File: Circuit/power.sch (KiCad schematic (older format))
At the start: 19 parts, among them Q202 FDN340P, Q203 FDN340P, SW1 ON/OFF, U201 CN3063, U202 MCP6002

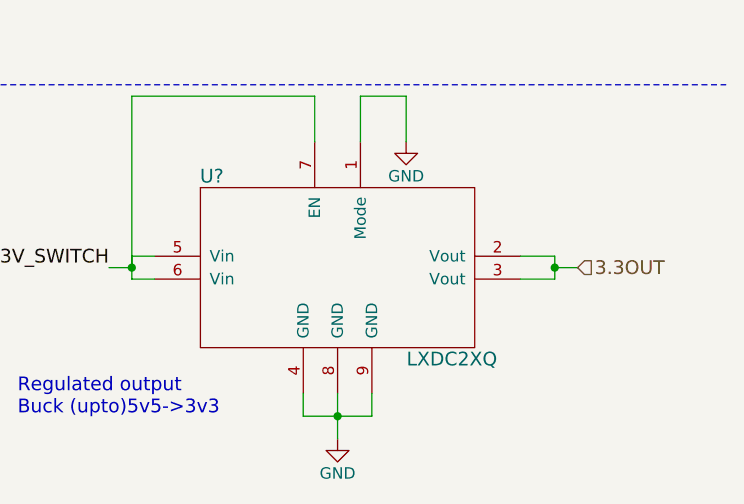
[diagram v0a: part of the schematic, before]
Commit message: Output cap on buck.
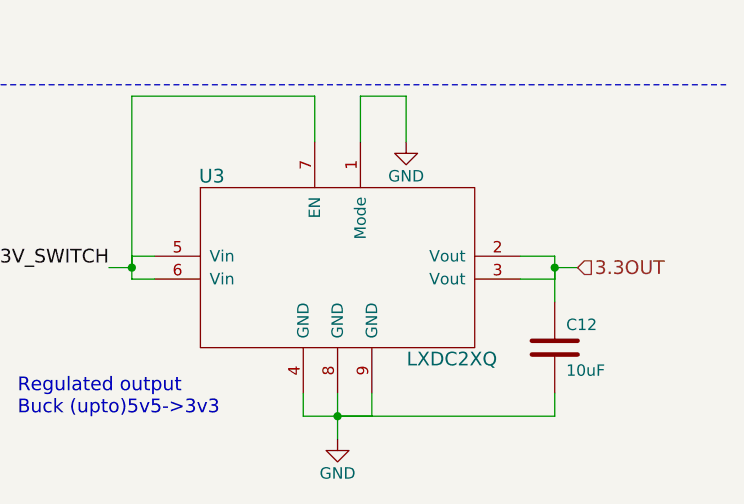
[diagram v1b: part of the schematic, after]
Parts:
- added C12: 10uF, symbol CAP
- gave numbers to parts that had none: 1
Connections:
- wire segments 74 -> 77
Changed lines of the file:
@@
 USB_IN
 $Comp
-L GND #PWR032
+L GND #PWR32
 U 1 1 563C4E24
 P 3950 4650
-F 0 "#PWR032" H 3950 4400 50  0001 C CNN
+F 0 "#PWR32" H 3950 4400 50  0001 C CNN
 F 1 "GND" H 3950 4500 50  0000 C CNN
 F 2 "" H 3950 4650 60  0000 C CNN
@@
 Charging current\nIr = 252mA max
 $Comp
-L GND #PWR033
+L GND #PWR35
 U 1 1 56417FB3
 P 7450 4200
-F 0 "#PWR033" H 7450 3950 50  0001 C CNN
+F 0 "#PWR35" H 7450 3950 50  0001 C CNN
 F 1 "GND" H 7450 4050 50  0000 C CNN
 F 2 "" H 7450 4200 60  0000 C CNN
@@
 3.3OUT
 $Comp
-L GND #PWR034
+L GND #PWR40
 U 1 1 5641AA9F
 P 10250 2500
-F 0 "#PWR034" H 10250 2250 50  0001 C CNN
+F 0 "#PWR40" H 10250 2250 50  0001 C CNN
 F 1 "GND" H 10250 2350 50  0000 C CNN
 F 2 "" H 10250 2500 60  0000 C CNN
@@
 $EndComp
 $Comp
-L GND #PWR035
+L GND #PWR36
 U 1 1 5642C1C1
 P 9050 4100
-F 0 "#PWR035" H 9050 3850 50  0001 C CNN
+F 0 "#PWR36" H 9050 3850 50  0001 C CNN
 F 1 "GND" H 9050 3950 50  0000 C CNN
 F 2 "" H 9050 4100 60  0000 C CNN
@@
 $EndComp
 $Comp
-L PWR_FLAG #FLG036
+L PWR_FLAG #FLG2
 U 1 1 5642D1CE
 P 10450 1800
-F 0 "#FLG036" H 10450 1895 50  0001 C CNN
+F 0 "#FLG2" H 10450 1895 50  0001 C CNN
 F 1 "PWR_FLAG" H 10450 1980 50  0000 C CNN
 F 2 "" H 10450 1800 60  0000 C CNN
@@
 $EndComp
 $Comp
-L PWR_FLAG #FLG037
+L PWR_FLAG #FLG1
 U 1 1 5642D5A3
 P 3900 1800
-F 0 "#FLG037" H 3900 1895 50  0001 C CNN
+F 0 "#FLG1" H 3900 1895 50  0001 C CNN
 F 1 "PWR_FLAG" H 3900 1980 50  0000 C CNN
 F 2 "" H 3900 1800 60  0000 C CNN
@@
 $EndComp
 $Comp
-L GND #PWR038
+L GND #PWR39
 U 1 1 5642DA26
 P 10000 4150
-F 0 "#PWR038" H 10000 3900 50  0001 C CNN
+F 0 "#PWR39" H 10000 3900 50  0001 C CNN
 F 1 "GND" H 10000 4000 50  0000 C CNN
 F 2 "" H 10000 4150 60  0000 C CNN
@@
 $EndComp
 $Comp
-L GND #PWR039
+L GND #PWR33
 U 1 1 5642CE9D
 P 4600 2350
-F 0 "#PWR039" H 4600 2100 50  0001 C CNN
+F 0 "#PWR33" H 4600 2100 50  0001 C CNN
 F 1 "GND" H 4600 2200 50  0000 C CNN
 F 2 "" H 4600 2350 60  0000 C CNN
@@
 $EndComp
 $Comp
-L GND #PWR040
+L GND #PWR34
 U 1 1 566FA00B
 P 6300 3100
-F 0 "#PWR040" H 6300 2850 50  0001 C CNN
+F 0 "#PWR34" H 6300 2850 50  0001 C CNN
 F 1 "GND" H 6300 2950 50  0000 C CNN
 F 2 "" H 6300 3100 60  0000 C CNN
@@
 Charge done not necessary? \nI'd just turn off the ~CHRG~ LED\n and call it good.
 $Comp
-L LXDC2XQ U?
+L LXDC2XQ U3
 U 1 1 5812C4CE
 P 9500 5550
-F 0 "U?" H 8950 5950 60  0000 C CNN
+F 0 "U3" H 8950 5950 60  0000 C CNN
 F 1 "LXDC2XQ" H 10000 5150 60  0000 C CNN
 F 2 "IoTuz:LXDC2XQ" H 9500 5550 60  0001 C CNN
@@
 $EndComp
 $Comp
-L GND #PWR?
+L GND #PWR37
 U 1 1 5812C93A
 P 9500 6300
-F 0 "#PWR?" H 9500 6050 50  0001 C CNN
+F 0 "#PWR37" H 9500 6050 50  0001 C CNN
 F 1 "GND" H 9500 6150 50  0000 C CNN
 F 2 "" H 9500 6300 60  0000 C CNN
@@
 $EndComp
 $Comp
-L GND #PWR?
+L GND #PWR38
 U 1 1 5812E212
 P 9800 5000
-F 0 "#PWR?" H 9800 4750 50  0001 C CNN
+F 0 "#PWR38" H 9800 4750 50  0001 C CNN
 F 1 "GND" H 9800 4850 50  0000 C CNN
 F 2 "" H 9800 5000 60  0000 C CNN
@@
 	1    0    0    -1
 $EndComp
+$Comp
+L CAP C12
+U 1 1 5812F47A
+P 10450 5900
+F 0 "C12" H 10500 6000 50  0000 L CNN
+F 1 "10uF" H 10500 5800 50  0000 L CNN
+F 2 "" H 10450 5900 60  0000 C CNN
+F 3 "" H 10450 5900 60  0000 C CNN
+	1    10450 5900
+	1    0    0    -1
+$EndComp
 Wire Wire Line
 	5050 3050 5050 2750
@@
 Wire Notes Line
 	7900 4750 11200 4750
+Wire Wire Line
+	10450 5550 10450 5700
+Wire Wire Line
+	10450 6100 10450 6200
+Wire Wire Line
+	10450 6200 9500 6200
 $EndSCHEMATC
